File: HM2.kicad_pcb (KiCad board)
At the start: 4 copper layers, 35 x 89.1 mm, 98 parts, among them J2 Barrel_Jack_MountingPin, Q1 2SK880, Q2 2SC2713, Q3 2SA1163, Q4 2SC2713, U1 TL072, U2 TL072, U3 TL072

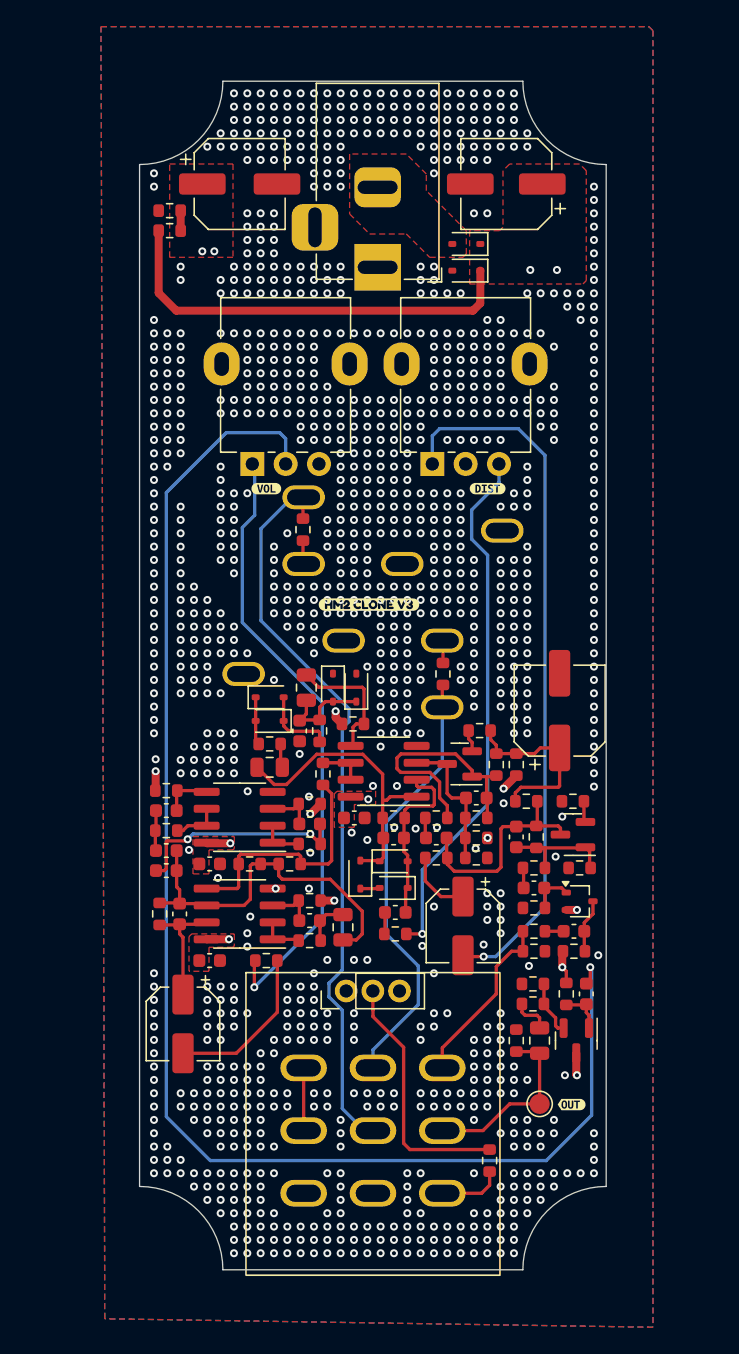
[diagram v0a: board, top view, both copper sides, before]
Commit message: V5 layout to review
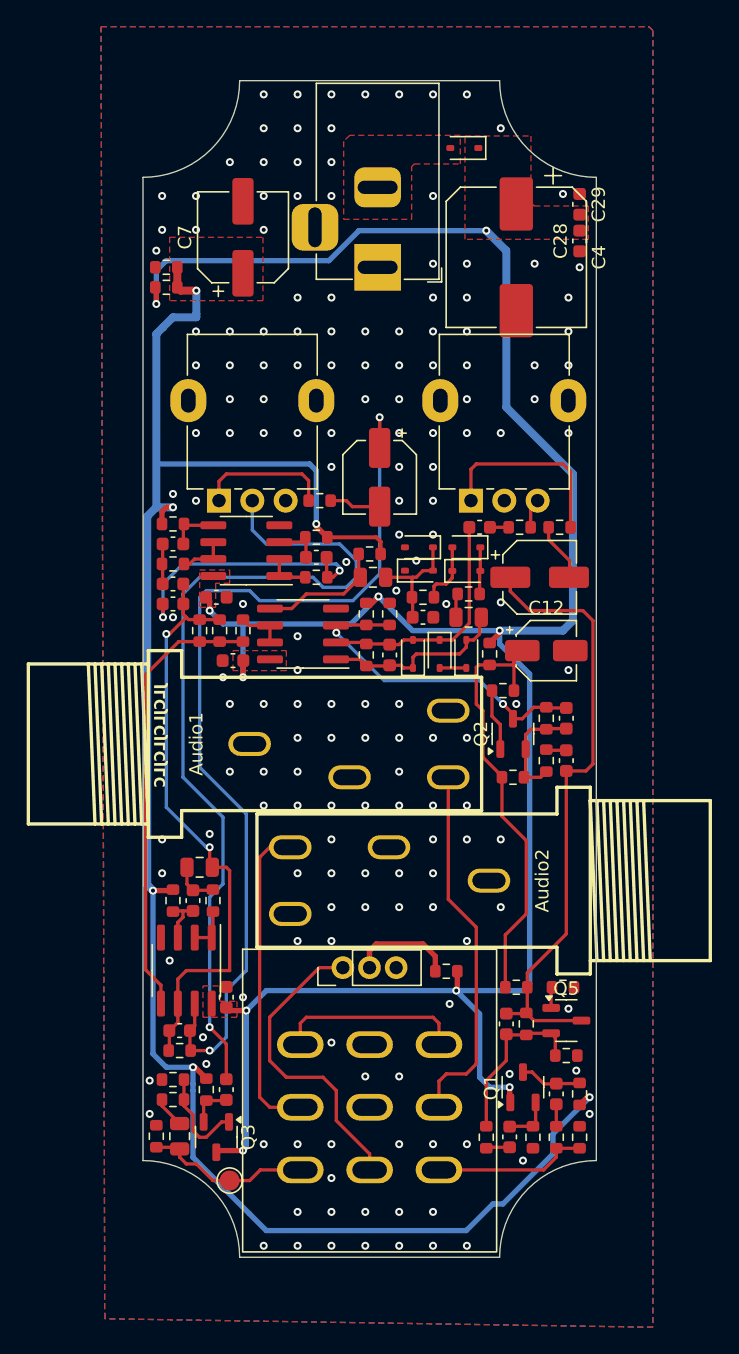
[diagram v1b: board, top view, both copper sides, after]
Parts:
- removed D2: 1N5819WS, Diode_SMD:D_SOD-323
- removed Q4: 2SC2713, Package_TO_SOT_SMD:SOT-23
- removed R39, R40: 0R, Resistor_SMD:R_0603_1608Metric
- removed kibuzzard-66C77FFB: G***, kibuzzard-66C77FFB
- removed kibuzzard-66C78013: G***, kibuzzard-66C78013
- removed kibuzzard-66C78027: G***, kibuzzard-66C78027
- removed kibuzzard-66C78076: G***, kibuzzard-66C78076
- removed kibuzzard-66C78083: G***, kibuzzard-66C78083
- removed kibuzzard-66C7864F: G***, kibuzzard-66C7864F
- added C28: 100n, Capacitor_SMD:C_0603_1608Metric, F.Cu at (217.0, 51.0)
- added C29: 10n, Capacitor_SMD:C_0603_1608Metric, F.Cu at (217.0, 48.3)
- added Q5: 2N3904, Package_TO_SOT_SMD:SOT-23-3, F.Cu at (216.0, 109.5)
- Audio1, Audio2: moved to F.Cu
- C12: footprint Capacitor_SMD:CP_Elec_6.3x5.4 -> Capacitor_SMD:CP_Elec_4x5.8
- C4: value 100u -> 470u; footprint Capacitor_SMD:CP_Elec_6.3x7.7 -> Capacitor_SMD:CP_Elec_10x10
- C7: footprint Capacitor_SMD:CP_Elec_6.3x5.4 -> Capacitor_SMD:CP_Elec_6.3x5.8
- Q1: value 2SK880 -> MMBFJ201; footprint Package_TO_SOT_SMD:SOT-323_SC-70 -> Package_TO_SOT_SMD:SOT-23-3
- Q2: value 2SC2713 -> 2N3906; footprint Package_TO_SOT_SMD:SOT-23 -> Package_TO_SOT_SMD:SOT-23-3
- Q3: value 2SA1163 -> 2N3904; footprint Package_TO_SOT_SMD:SOT-23 -> Package_TO_SOT_SMD:SOT-23-3
- R32: value 470k -> 220k
- moved C18 43.6 mm to (202.0, 68.8)
- moved R31 34.7 mm to (197.5, 70.5)
- moved Q3 33.4 mm to (189.8, 118.2), turned to -90 degrees
- moved R22 31.9 mm to (212.5, 72.5)
- moved C15 29.6 mm to (209.5, 72.5), turned to 180 degrees
- moved C20 27.9 mm to (190.5, 114.7)
- moved C22 27.9 mm to (187.0, 118.2)
- moved R33 27.9 mm to (189.0, 114.7)
- moved R34 27.9 mm to (186.5, 113.9)
- moved R36 27.9 mm to (186.5, 115.4)
- moved R37 27.9 mm to (185.2, 118.2)
- moved C13 26.8 mm to (214.0, 76.2), turned to 0 degrees
- moved R20 26.5 mm to (215.5, 72.5), turned to 180 degrees
- moved TP1 24.0 mm to (190.8, 121.5)
- moved R14 20.5 mm to (210.0, 118.2), turned to 90 degrees
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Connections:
- Audio1 pad 4: Net-(Audio1-Pad4) -> /IN
- Audio1 pad 5: /OUT -> GND
- Audio2 pad 4: Net-(Audio2-Pad4) -> /OUT
- Audio2 pad 5: /IN -> GND
- C13 pad 1: Net-(C13-Pad1) -> Net-(Q5-C)
- C14 pad 1: Net-(Q2-C) -> Net-(Q5-C)
- C17 pad 1: Net-(Q3-C) -> Net-(Q2-C)
- C17 pad 2: Net-(Q3-B) -> Net-(Q2-B)
- C20 pad 1: Net-(Q4-B) -> Net-(Q3-B)
- C8 pad 1: Net-(Q1-S) -> Net-(Q1-D)
- C9 pad 1: Net-(Q2-B) -> Net-(Q5-B)
- C9 pad 2: Net-(Q2-C) -> Net-(Q5-C)
- Q1 pad 1: Net-(Q1-S) -> +9V
- Q1 pad 2: +9V -> Net-(Q1-D)
- Q2 pad 1: Net-(Q2-B) -> Net-(Q2-E)
- Q2 pad 2: Net-(Q2-E) -> Net-(Q2-B)
- Q3 pad 1: Net-(Q3-B) -> Net-(Q3-E)
- Q3 pad 2: Net-(Q3-E) -> Net-(Q3-B)
- Q3 pad 3: Net-(Q3-C) -> +9V
- R10 pad 1: Net-(Q1-S) -> Net-(Q1-D)
- R14 pad 2: Net-(Q2-B) -> Net-(Q5-B)
- R15 pad 2: Net-(Q2-B) -> Net-(Q5-B)
- R16 pad 1: Net-(Q2-C) -> Net-(Q5-C)
- R16 pad 2: Net-(Q2-B) -> Net-(Q5-B)
- R18 pad 2: Net-(Q2-C) -> Net-(Q5-C)
- R19 pad 2: Net-(Q2-E) -> Net-(Q5-E)
- R20 pad 1: Net-(C13-Pad1) -> Net-(R20-Pad1)
- R20 pad 2: Net-(Q2-C) -> Net-(C13-Pad2)
- R23 pad 2: Net-(Q3-B) -> Net-(Q2-B)
- R24 pad 2: Net-(Q3-B) -> Net-(Q2-B)
- R26 pad 1: Net-(Q3-C) -> Net-(Q2-C)
- R26 pad 2: Net-(Q3-B) -> Net-(Q2-B)
- R28 pad 1: Net-(Q3-E) -> Net-(Q2-E)
- R29 pad 2: Net-(Q3-C) -> Net-(Q2-C)
- R30 pad 1: Net-(Q3-C) -> Net-(Q2-C)
- R33 pad 2: Net-(Q4-B) -> Net-(Q3-B)
- R34 pad 1: Net-(Q4-E) -> Net-(Q3-E)
- R36 pad 1: Net-(Q4-E) -> Net-(Q3-E)
- R8 pad 1: /IN_LED -> +9V
- RV3 pad 1: Net-(C13-Pad2) -> Net-(R20-Pad1)
- SW1 pad 10: (no net) -> /GND_LED
- SW1 pad 12: GND -> (no net)
- SW1 pad 2: Net-(SW1-A-Pad1) -> /OUT
- SW1 pad 3: unconnected-(SW1-A-Pad3) -> /OUT_FX
- SW1 pad 4: /IN -> GND
- SW1 pad 5: /OUT -> GND
- SW1 pad 6: +9V -> /GND_LED
- SW1 pad 7: /IN_FX -> Net-(SW1-A-Pad1)
- SW1 pad 8: /OUT_FX -> /IN
- SW1 pad 9: /IN_LED -> /IN_FX
- U1 pad 3: Net-(Q3-C) -> Net-(Q2-C)
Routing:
- net Net-(C16-Pad1): track 8.98 -> 70.8 mm, vias 0 -> 2
- net Net-(C13-Pad2): track 53.2 -> 4.42 mm, vias 1 -> 0
- net Net-(Q5-C): track 0.00 -> 46.4 mm
- net Net-(C20-Pad2): track 106.9 -> 64.9 mm
- net Net-(R22-Pad2): track 39.8 -> 2.22 mm, vias 1 -> 0
- net Net-(R31-Pad1): track 46.3 -> 10.1 mm, vias 1 -> 0
- net /OUT: track 56.0 -> 24.0 mm
- net /GND_LED: track 0.00 -> 23.2 mm
- net Net-(C12-Pad1): track 13.8 -> 32.8 mm
- net Net-(U2B--): track 27.4 -> 45.0 mm, vias 0 -> 2
- net /+4V5: track 122.6 -> 139.9 mm, vias 7 -> 6
- net Net-(Q3-B): track 19.1 -> 3.20 mm
- net Net-(U2B-+): track 18.5 -> 33.5 mm
- net Net-(R20-Pad1): track 0.00 -> 14.4 mm
- net Net-(Q5-B): track 0.00 -> 12.8 mm
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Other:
- board size 35 x 89.1 mm -> 34 x 88.2 mm
